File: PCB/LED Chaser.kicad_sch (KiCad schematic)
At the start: 18 parts, among them J1 Conn_01x03_Pin, U1 NE555P, U2 4017

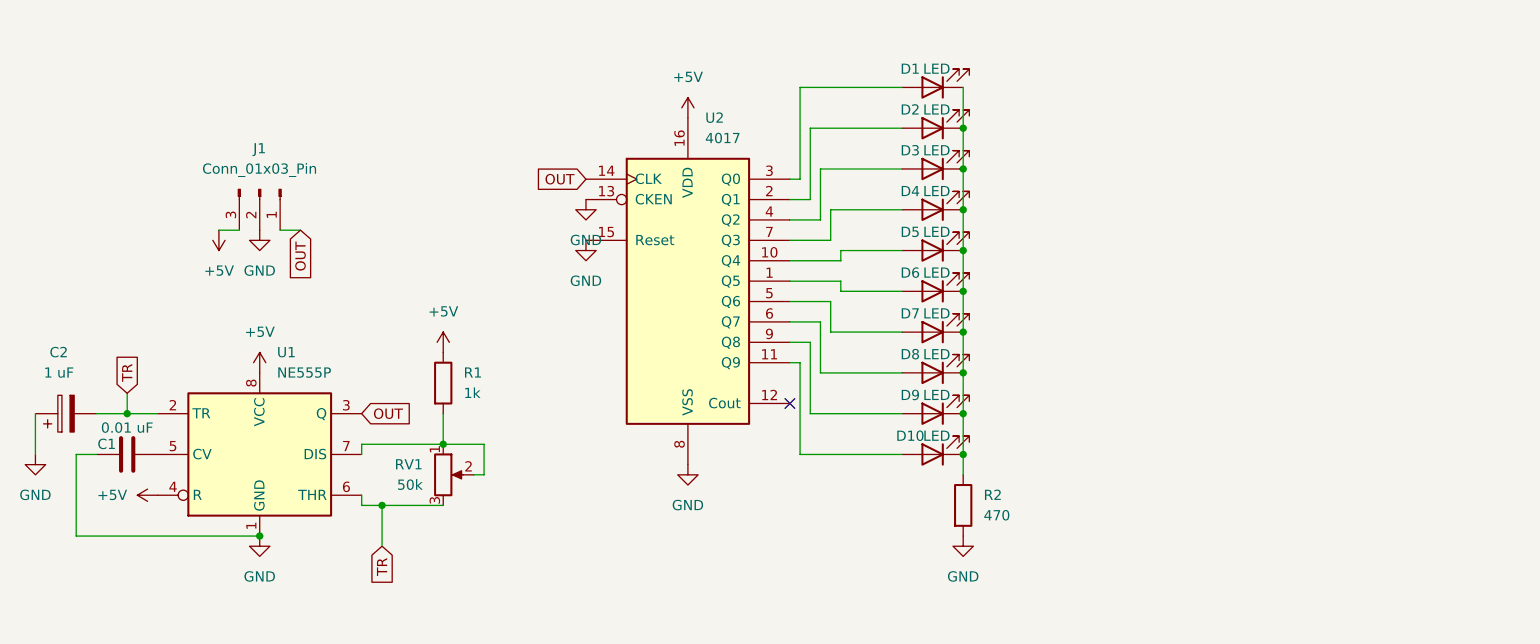
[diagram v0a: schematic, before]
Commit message: cleaned up schematic and updated readme
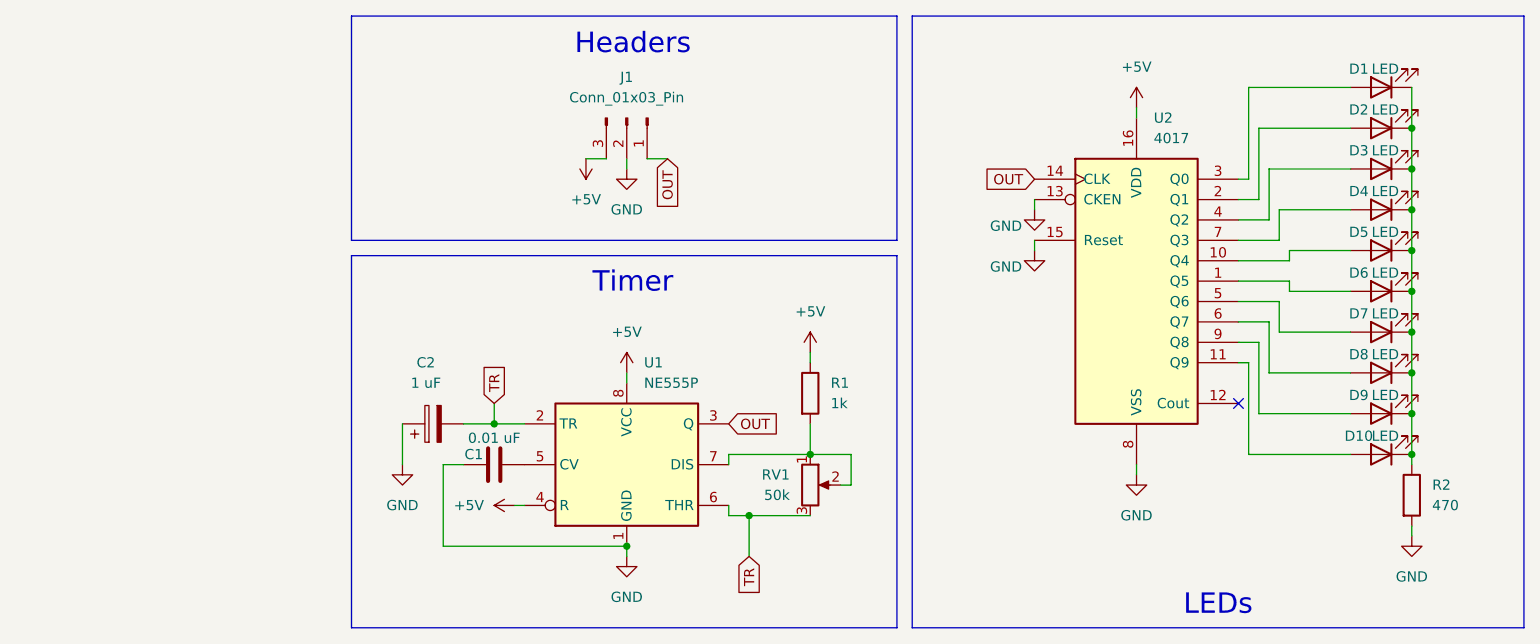
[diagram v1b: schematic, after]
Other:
- note added: "Headers"
- note added: "LEDs"
- note added: "Timer"
- moved on the sheet: C1, C2, D1, D10, D2, D3, D4, D5, D6, D7, D8, D9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
